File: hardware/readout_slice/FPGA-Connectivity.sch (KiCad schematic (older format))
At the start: 24 parts

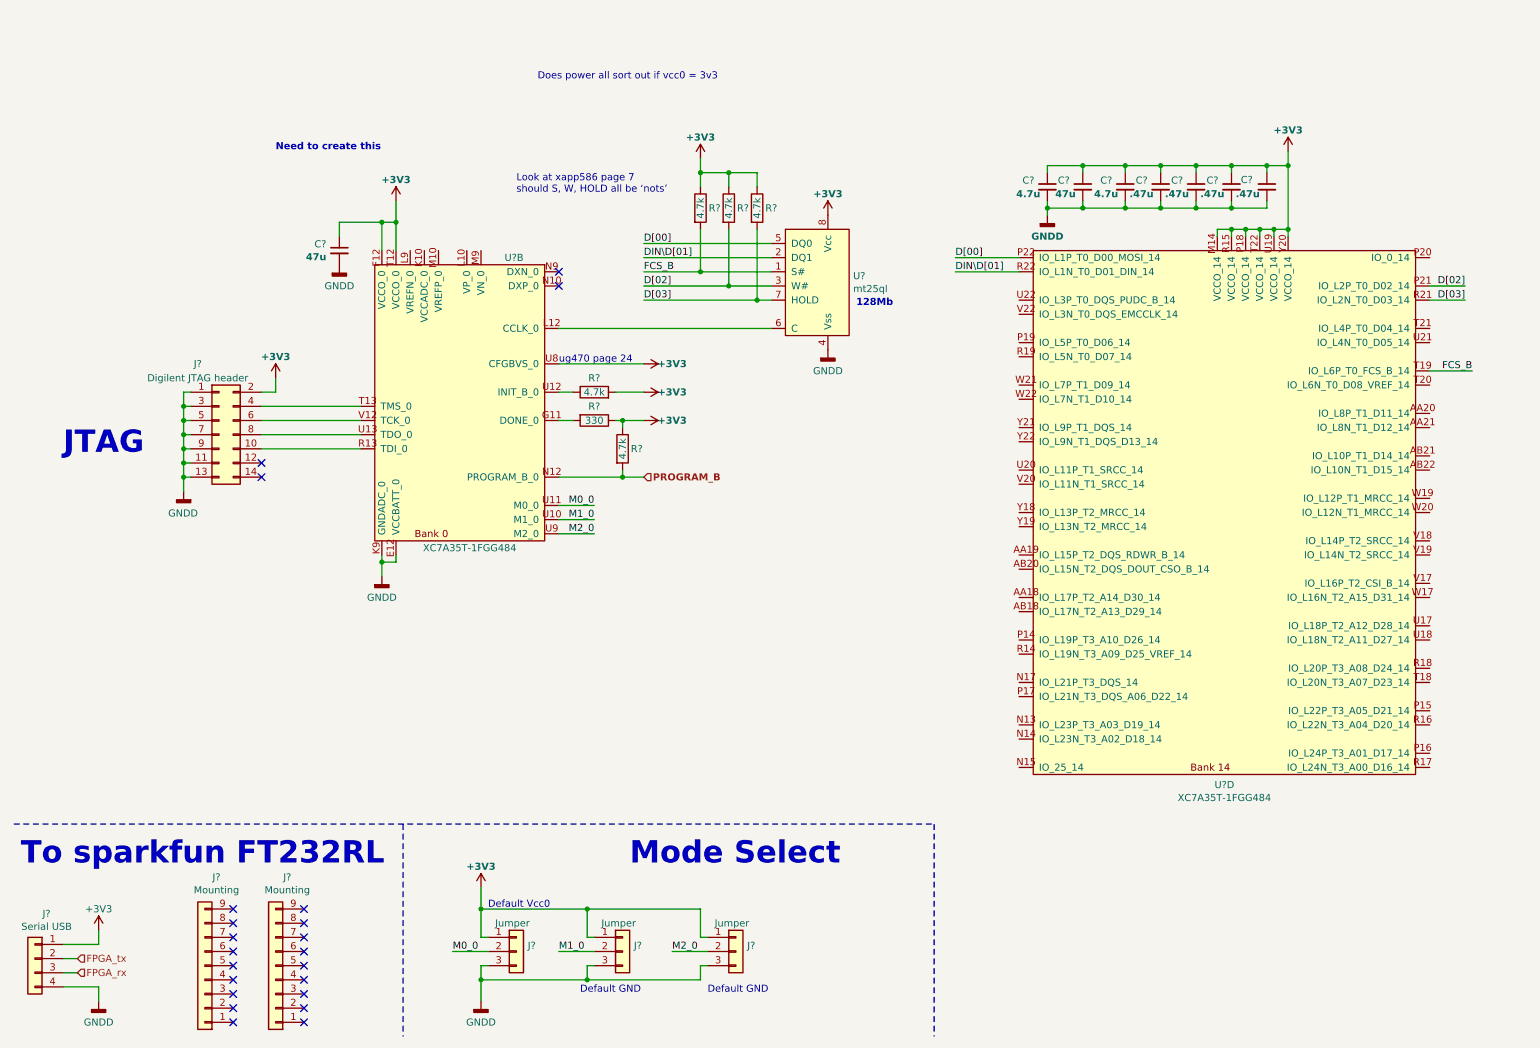
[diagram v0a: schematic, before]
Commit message: auto push run at Wed Apr 21 11:14:23 EDT 2021
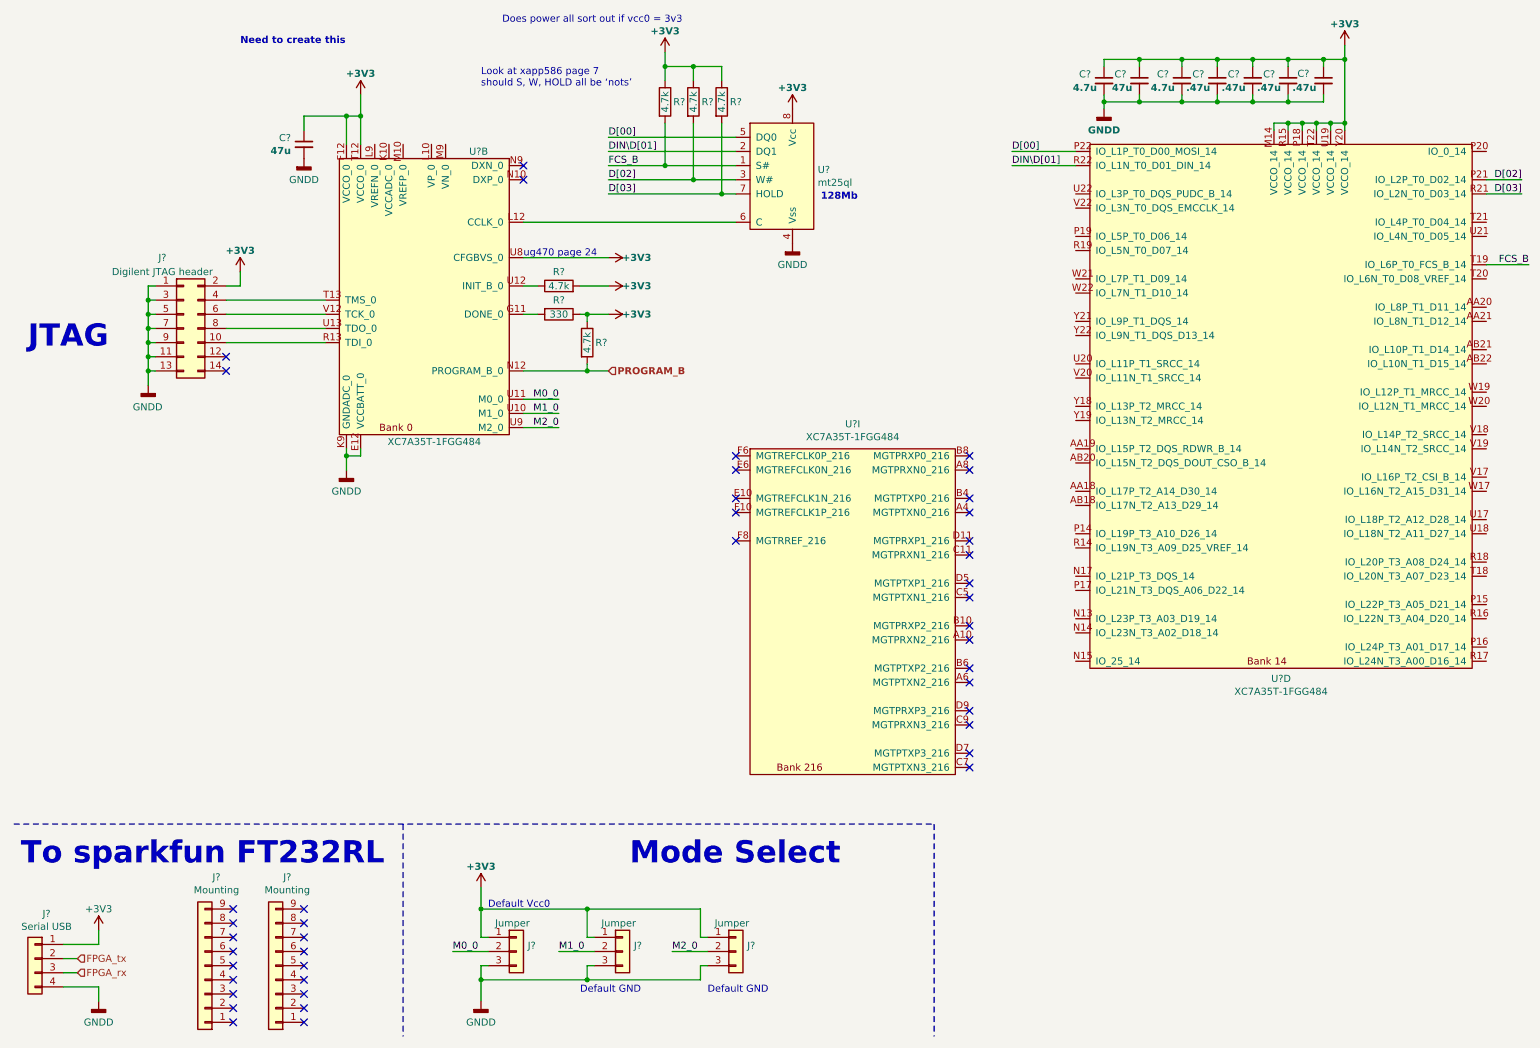
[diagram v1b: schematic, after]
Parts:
- added U?: XC7A35T-1FGG484, symbol readout:XC7A35T-1FGG484
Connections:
- no-connect marks 22 -> 43
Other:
- moved on the sheet: C?, J?, R?, U?, U?B, U?D
